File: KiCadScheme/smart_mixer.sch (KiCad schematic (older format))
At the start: 6 parts

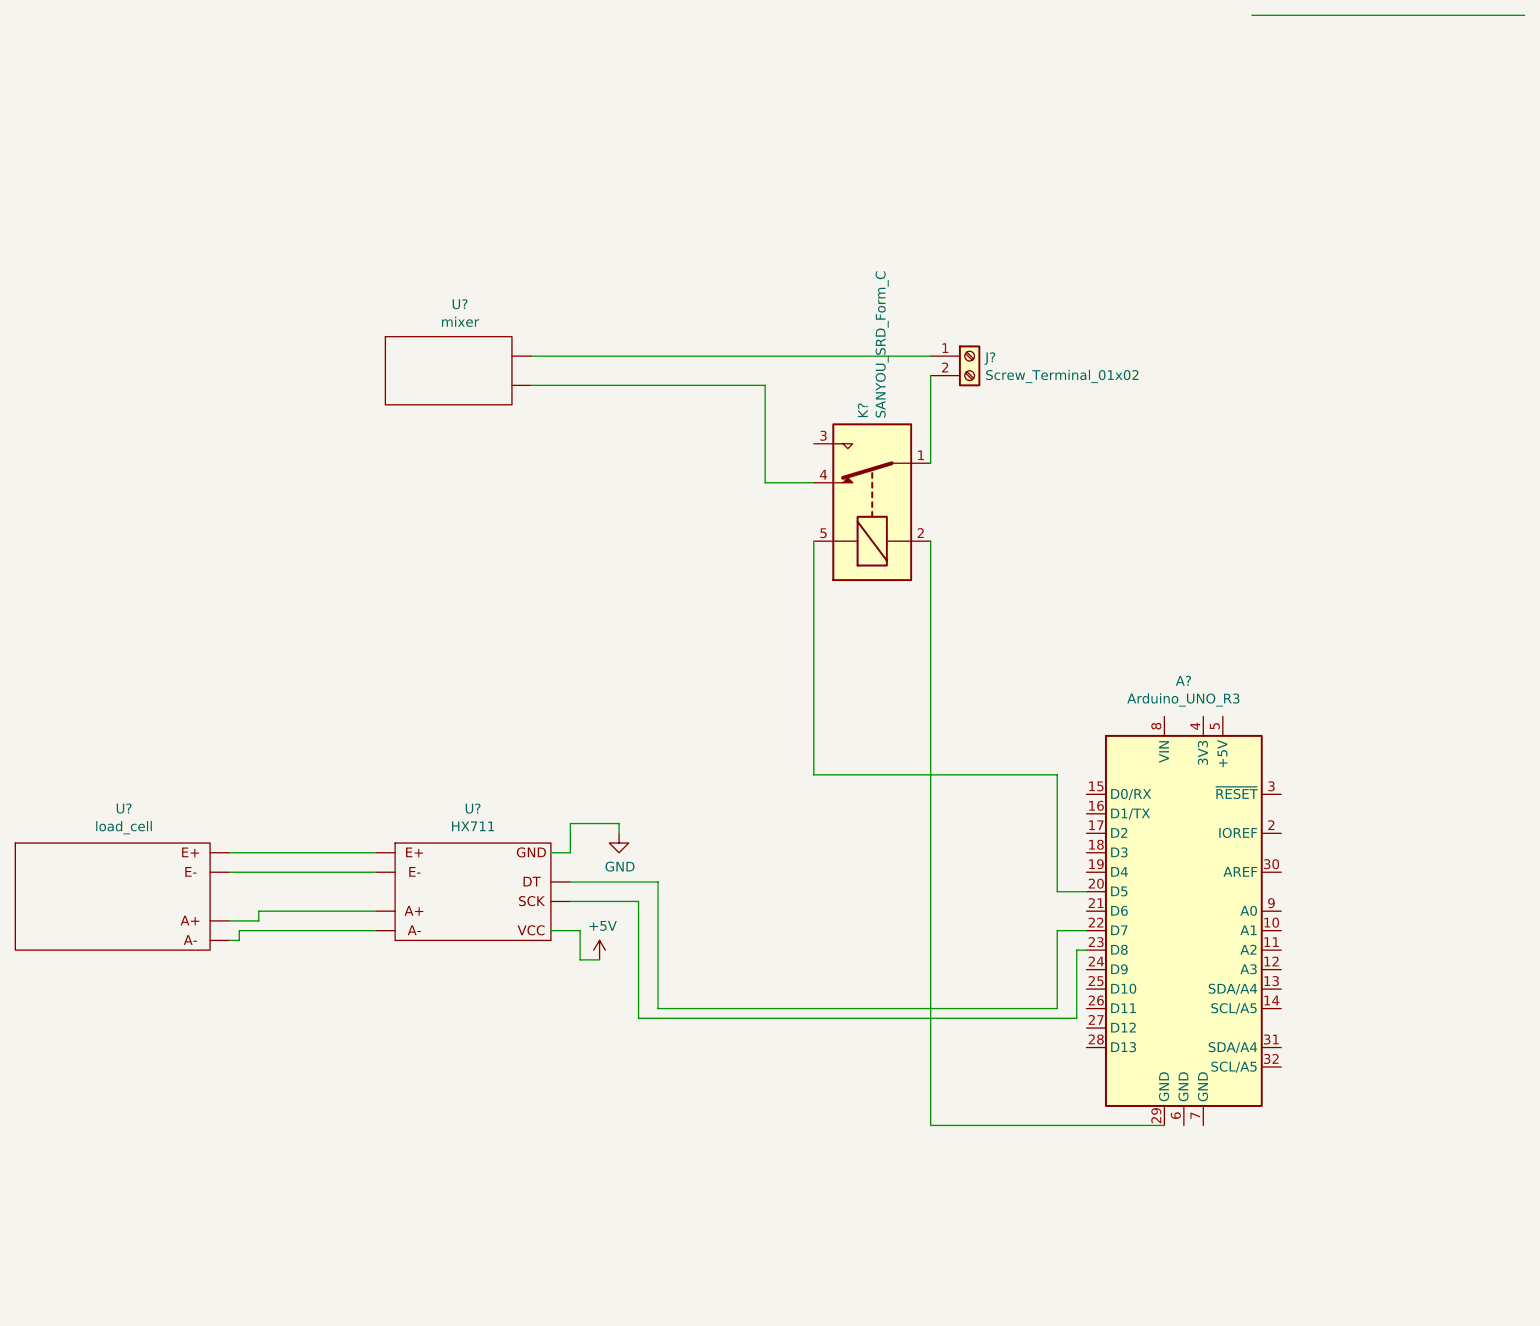
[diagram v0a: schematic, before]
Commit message: ss&m
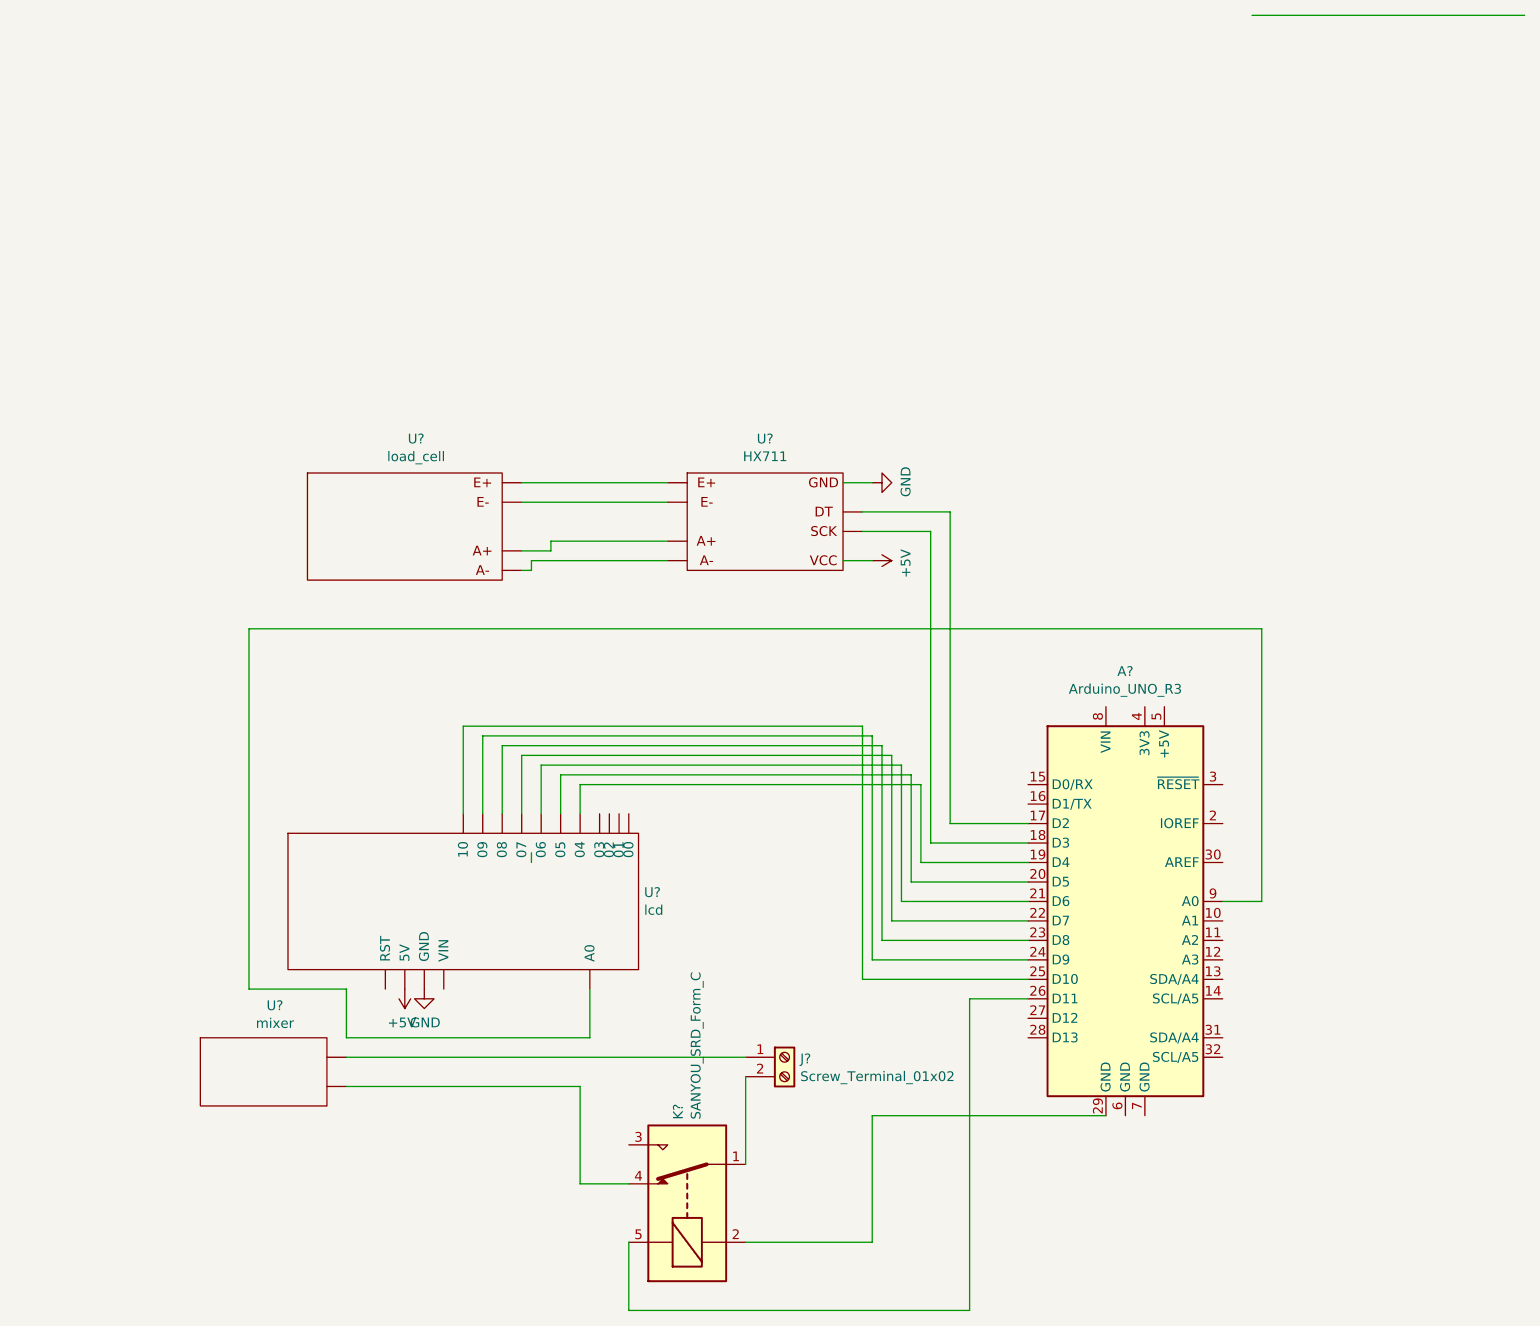
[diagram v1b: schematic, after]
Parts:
- added U?: lcd, symbol arduino_sen:lcd
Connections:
- wire segments 37 -> 66
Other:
- moved on the sheet: A?, J?, K?, U?
